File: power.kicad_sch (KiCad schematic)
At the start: 33 parts, among them J3 BATTERY, J5 USB_C_Receptacle_USB2.0_16P, SW20 POWER_BUTTON, U4 BQ21040DBV, U6 RT8059

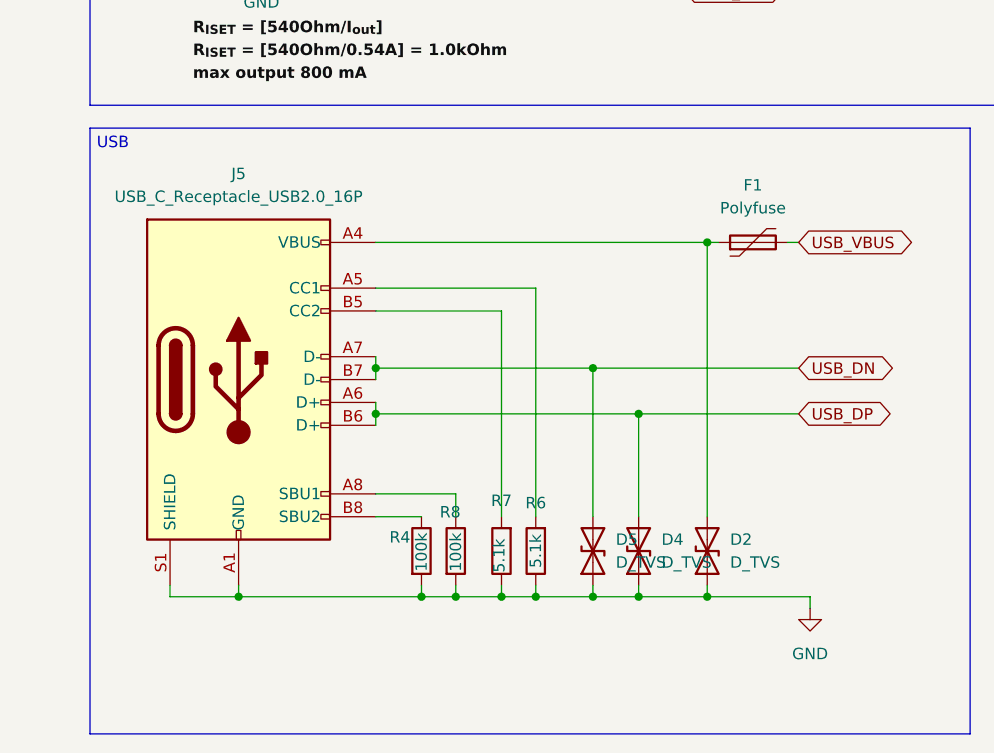
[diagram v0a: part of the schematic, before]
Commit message: lol
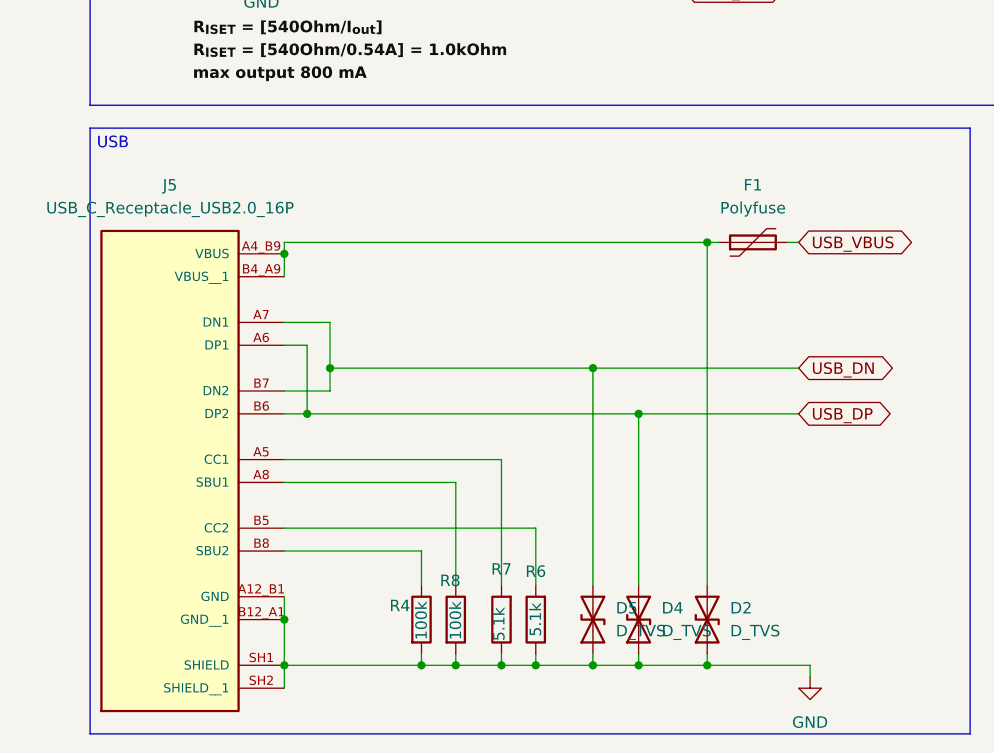
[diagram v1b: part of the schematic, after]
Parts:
- J5: symbol Connector:USB_C_Receptacle_USB2.0_16P -> UJ20-C-G-MSMT-TR-68:UJ20-C-G-MSMT-TR-68; MANUFACTURER (none) -> CUI Devices; PARTREV (none) -> 1.0; STANDARD (none) -> Manufacturer Recommendations
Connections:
- net GND: now also J5.A12_B1 (GND), J5.B12_A1 (GND__1), J5.SH1 (SHIELD), J5.SH2 (SHIELD__1); no longer J5.A1 (GND), J5.A12 (GND), J5.B1 (GND), J5.B12 (GND), J5.S1 (SHIELD)
- net at R6.2: now also J5.B5 (CC2); no longer J5.A5 (CC1)
- net at R7.2: now also J5.A5 (CC1); no longer J5.B5 (CC2)
- new net: D2.2 (A2), F1.1, J5.A4_B9 (VBUS), J5.B4_A9 (VBUS__1)
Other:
- moved on the sheet: D2, D4, D5, R4, R6, R7, R8
